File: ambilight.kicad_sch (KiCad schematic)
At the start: 21 parts, among them J1 RGB Connector, J3 USB4085-GF-A, SW1 RESET, SW2 BOOT, U2 ESP32-C3-MINI-1-H4, U4 AZ1117CR-3.3TRG1

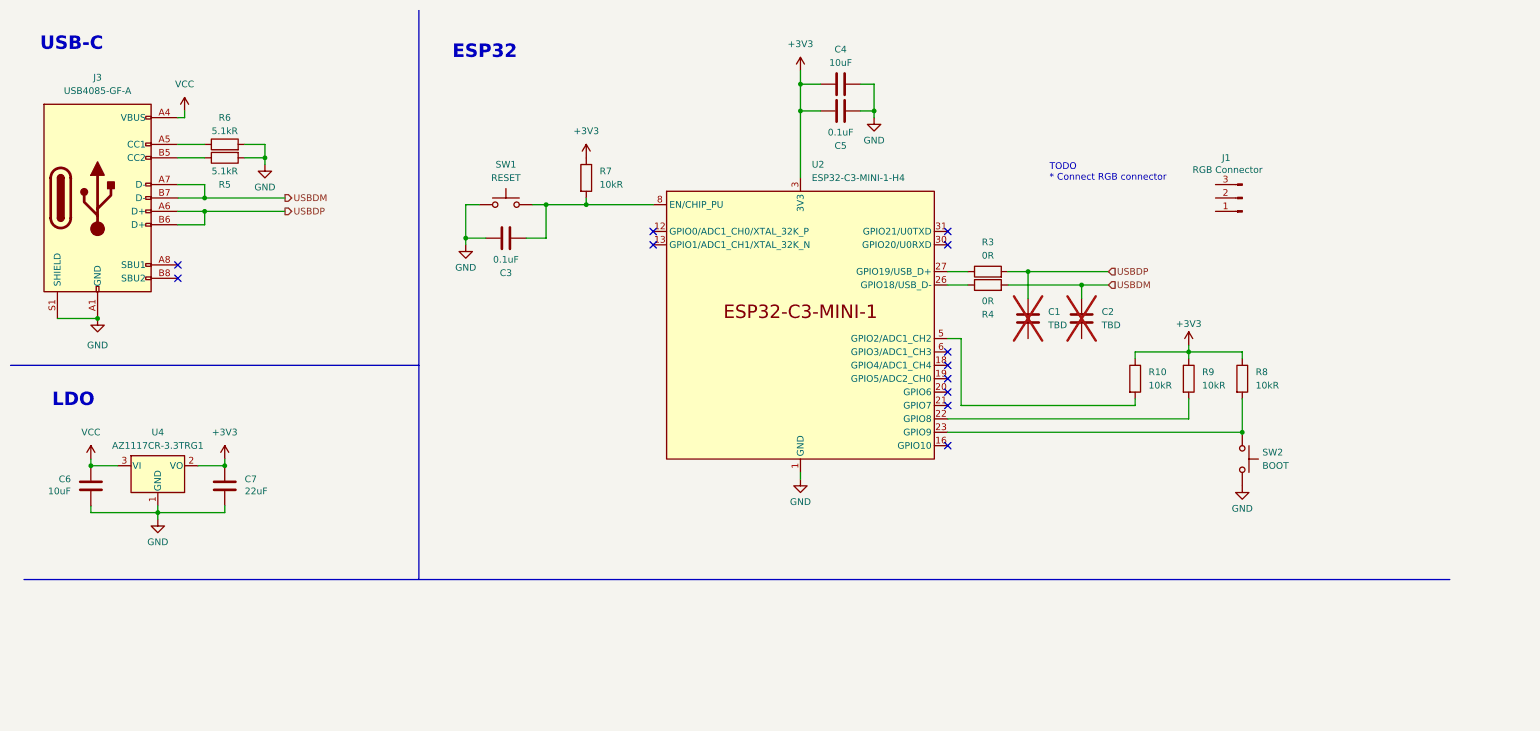
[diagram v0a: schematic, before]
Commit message: Bunch of updates and beginning of PCB layout
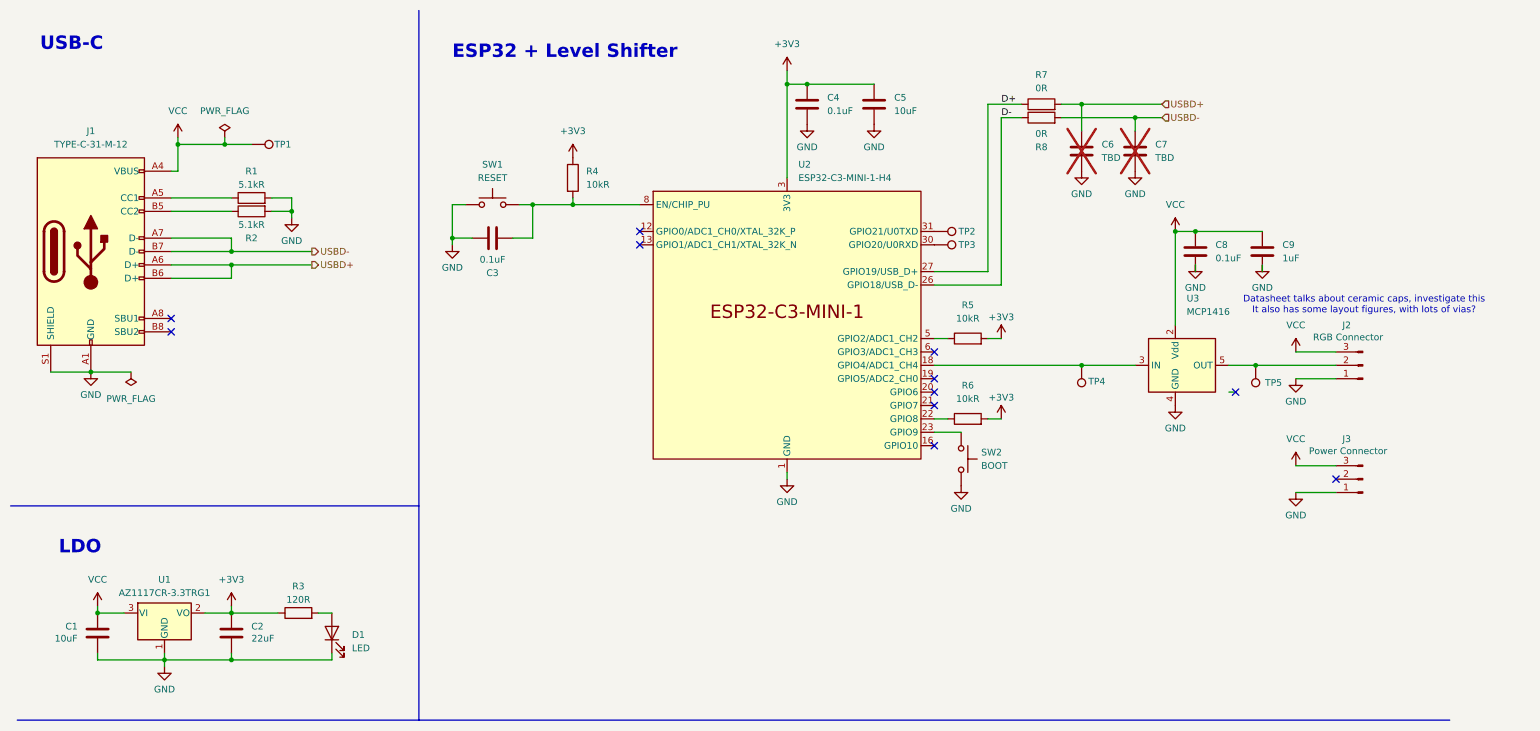
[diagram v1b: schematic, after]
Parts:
- removed R8, R9: 10kR, symbol Device:R
- added C8: 0.1uF, Capacitor_SMD:C_0805_2012Metric, symbol Device:C
- added C9: 1uF, Capacitor_SMD:C_0805_2012Metric, symbol Device:C
- added D1: LED, LED_SMD:LED_0805_2012Metric, symbol Device:LED
- added J3: Power Connector, Connector_PinHeader_2.54mm:PinHeader_1x03_P2.54mm_Vertical, symbol Connector:Conn_01x03_Pin
- added R3: 120R, Resistor_SMD:R_0805_2012Metric, symbol Device:R
- added R6: 10kR, Resistor_SMD:R_0805_2012Metric, symbol Device:R
- added TP1, TP2, TP3, TP4, TP5: ~, Custom_PCBWay:TestPoint_Pad_D2.5mm_SilkscreenFix, symbol Connector:TestPoint
- added U3: MCP1416, Package_TO_SOT_SMD:SOT-23-5, symbol Driver_FET:MCP1416
- C1: renamed from C6; footprint (none) -> Capacitor_SMD:C_0805_2012Metric
- C2: renamed from C7; footprint (none) -> Capacitor_SMD:C_0805_2012Metric
- C3: footprint (none) -> Capacitor_SMD:C_0805_2012Metric
- C4: value 10uF -> 0.1uF; footprint (none) -> Capacitor_SMD:C_0805_2012Metric
- C5: value 0.1uF -> 10uF; footprint (none) -> Capacitor_SMD:C_0805_2012Metric
- C6: renamed from C1; footprint (none) -> Capacitor_SMD:C_0805_2012Metric
- C7: renamed from C2; footprint (none) -> Capacitor_SMD:C_0805_2012Metric
- J1: renamed from J3; value USB4085-GF-A -> TYPE-C-31-M-12; footprint Connector_USB:USB_C_Receptacle_GCT_USB4085 -> Connector_USB:USB_C_Receptacle_HRO_TYPE-C-31-M-12
- R1: renamed from R6; footprint (none) -> Resistor_SMD:R_0805_2012Metric
- R2: renamed from R5; footprint (none) -> Resistor_SMD:R_0805_2012Metric
- R4: renamed from R7; footprint (none) -> Resistor_SMD:R_0805_2012Metric
- R5: renamed from R10; footprint (none) -> Resistor_SMD:R_0805_2012Metric
- R7: renamed from R3; footprint (none) -> Resistor_SMD:R_0805_2012Metric
- R8: renamed from R4; footprint (none) -> Resistor_SMD:R_0805_2012Metric
- SW1, SW2: footprint (none) -> Button_Switch_SMD:SW_Push_1P1T_NO_CK_KMR2
- renumbered J1 to J2, U4 to U1
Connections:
- net +3V3: now also C4.1, C5.1, R5.2, R3.1, R6.2; no longer C4.2, C5.2, R5.1
- net GND: now also C4.2, C5.2, C6.2, C7.2, J2.1 (Pin_1), C8.2, C9.2, D1.1 (K), J3.1 (Pin_1), U3.4 (GND); no longer C4.1, C5.1
- net VCC: now also J2.3 (Pin_3), C8.1, C9.1, J3.3 (Pin_3), TP1.1, U3.2 (Vdd)
- net at U2.18 (GPIO4/ADC1_CH4): now also TP4.1, U3.3 (IN)
- net at U2.22 (GPIO8): now also R6.1
- net D-: now reaches R8.1, U2.26 (GPIO18/USB_D-)
- net D+: now reaches R7.1, U2.27 (GPIO19/USB_D+)
- net at U2.30 (GPIO20/U0RXD): now also TP3.1
- net at U2.31 (GPIO21/U0TXD): now also TP2.1
- net at U2.5 (GPIO2/ADC1_CH2): now also R5.1; no longer R5.2
- net at J2.2 (Pin_2): now also TP5.1, U3.5 (OUT)
- net USBDM renamed USBD-
- net USBDP renamed USBD+
- new net: D1.2 (A), R3.2
- no-connect marks 12 -> 11
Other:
- note added: "Datasheet talks about ceramic caps, investigate this It also has some layout figures, with lots of vias?"
- note added: "ESP32 + Level Shifter"
- note removed: "ESP32"
- note removed: "TODO * Connect RGB connector"
- moved on the sheet: C1, C2, C3, C6, C7, J1, J2, R1, R2, R4, R5, R7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
